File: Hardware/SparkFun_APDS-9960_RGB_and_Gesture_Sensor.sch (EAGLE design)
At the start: 19 parts, among them U1 APDS-9960

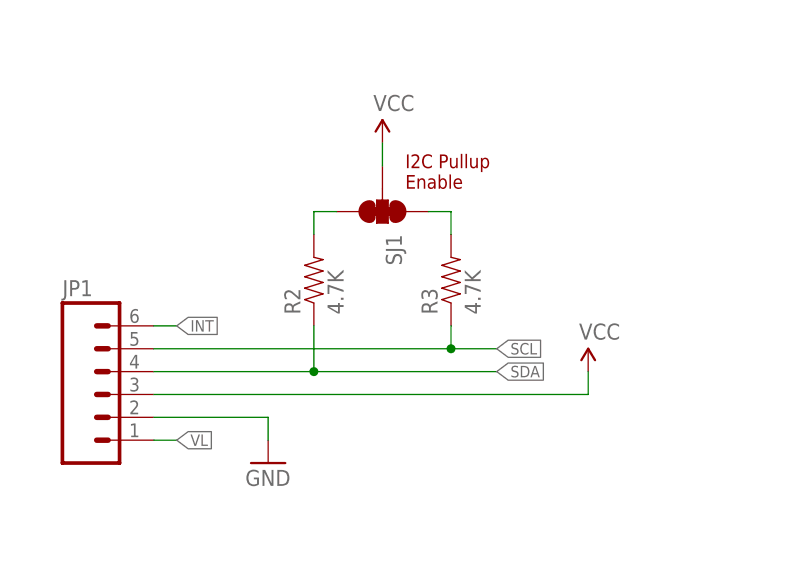
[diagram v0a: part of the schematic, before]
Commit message: Reverting to current board layout files
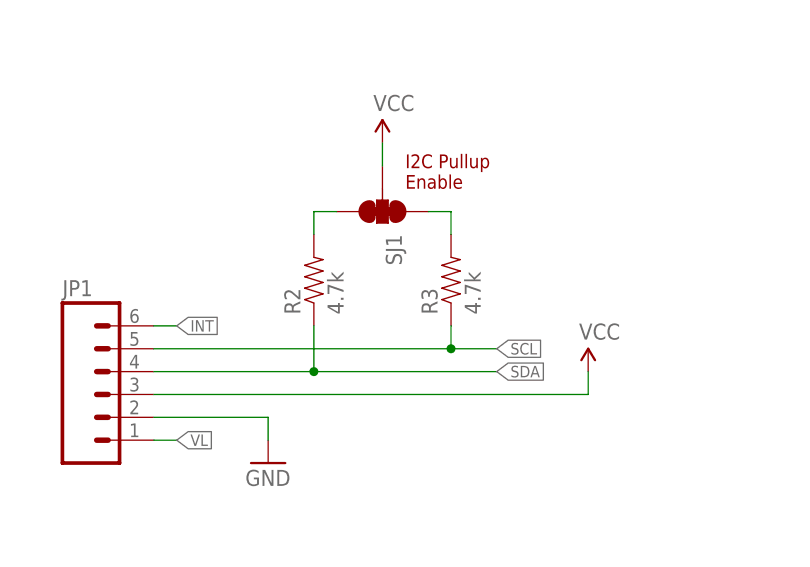
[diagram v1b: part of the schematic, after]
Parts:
- R2, R3: value 4.7K -> 4.7k; device SparkFun-Resistors:4.7KOHM-1/10W-1%(0603) -> SparkFun-Resistors:4.7KOHM1/10W1%(0603)
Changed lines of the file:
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@@
 <?xml version="1.0" encoding="utf-8"?>
 <!DOCTYPE eagle SYSTEM "eagle.dtd">
-<eagle version="7.2.0">
+<eagle version="6.5.0">
 <drawing>
 <settings>
@@
 <layer number="254" name="cooling" color="7" fill="1" visible="yes" active="yes"/>
 </layers>
-<schematic xreflabel="%F%N/%S" xrefpart="/%S.%C%R">
+<schematic xreflabel="%F%N/%S.%C%R" xrefpart="/%S.%C%R">
 <attributes>
 </attributes>
@@
 <part name="GND1" library="SparkFun-Aesthetics" deviceset="GND" device=""/>
 <part name="R1" library="SparkFun-Resistors" deviceset="10KOHM1/10W1%(0603)" device="0603" value="10k"/>
-<part name="R2" library="SparkFun-Resistors" deviceset="4.7KOHM-1/10W-1%(0603)" device="" value="4.7K"/>
+<part name="R2" library="SparkFun-Resistors" deviceset="4.7KOHM1/10W1%(0603)" device="" value="4.7k"/>
 <part name="SJ1" library="SparkFun-Passives" deviceset="SOLDERJUMPER_2WAY" device="PASTE1&amp;2&amp;3"/>
 <part name="SUPPLY2" library="SparkFun-Aesthetics" deviceset="VCC" device=""/>
@@
 <part name="LOGO2" library="SparkFun-Aesthetics" deviceset="OSHW-LOGO" device="S"/>
 <part name="R4" library="SparkFun-Resistors" deviceset="RESISTOR" device="0603" value="DNP"/>
-<part name="R3" library="SparkFun-Resistors" deviceset="4.7KOHM-1/10W-1%(0603)" device="" value="4.7K"/>
+<part name="R3" library="SparkFun-Resistors" deviceset="4.7KOHM1/10W1%(0603)" device="" value="4.7k"/>
 <part name="SJ2" library="SparkFun-Retired" deviceset="SOLDERJUMPER" device="NC"/>
 <part name="C1" library="SparkFun-Capacitors" deviceset="100UF-10V-10%(TANT)" device="" value="100uF"/>

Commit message: Changed 4.7k resistors to proper 0603-RES package.
This adds a small silkscreen dot under the resistor.
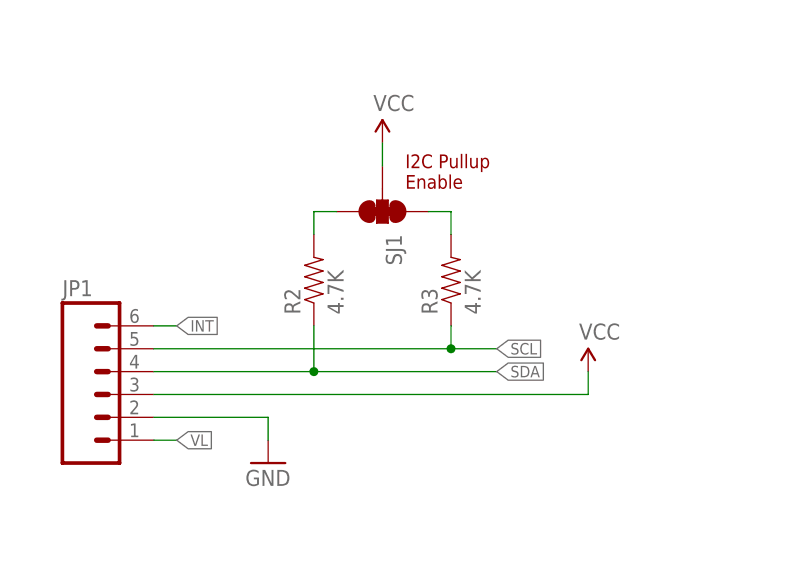
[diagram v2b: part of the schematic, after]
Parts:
- R2, R3: value 4.7k -> 4.7K; device SparkFun-Resistors:4.7KOHM1/10W1%(0603) -> SparkFun-Resistors:4.7KOHM-1/10W-1%(0603)
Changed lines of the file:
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@@
 <?xml version="1.0" encoding="utf-8"?>
 <!DOCTYPE eagle SYSTEM "eagle.dtd">
-<eagle version="6.5.0">
+<eagle version="7.2.0">
 <drawing>
 <settings>
@@
 <layer number="254" name="cooling" color="7" fill="1" visible="yes" active="yes"/>
 </layers>
-<schematic xreflabel="%F%N/%S.%C%R" xrefpart="/%S.%C%R">
+<schematic xreflabel="%F%N/%S" xrefpart="/%S.%C%R">
 <attributes>
 </attributes>
@@
 <part name="GND1" library="SparkFun-Aesthetics" deviceset="GND" device=""/>
 <part name="R1" library="SparkFun-Resistors" deviceset="10KOHM1/10W1%(0603)" device="0603" value="10k"/>
-<part name="R2" library="SparkFun-Resistors" deviceset="4.7KOHM1/10W1%(0603)" device="" value="4.7k"/>
+<part name="R2" library="SparkFun-Resistors" deviceset="4.7KOHM-1/10W-1%(0603)" device="" value="4.7K"/>
 <part name="SJ1" library="SparkFun-Passives" deviceset="SOLDERJUMPER_2WAY" device="PASTE1&amp;2&amp;3"/>
 <part name="SUPPLY2" library="SparkFun-Aesthetics" deviceset="VCC" device=""/>
@@
 <part name="LOGO2" library="SparkFun-Aesthetics" deviceset="OSHW-LOGO" device="S"/>
 <part name="R4" library="SparkFun-Resistors" deviceset="RESISTOR" device="0603" value="DNP"/>
-<part name="R3" library="SparkFun-Resistors" deviceset="4.7KOHM1/10W1%(0603)" device="" value="4.7k"/>
+<part name="R3" library="SparkFun-Resistors" deviceset="4.7KOHM-1/10W-1%(0603)" device="" value="4.7K"/>
 <part name="SJ2" library="SparkFun-Retired" deviceset="SOLDERJUMPER" device="NC"/>
 <part name="C1" library="SparkFun-Capacitors" deviceset="100UF-10V-10%(TANT)" device="" value="100uF"/>
